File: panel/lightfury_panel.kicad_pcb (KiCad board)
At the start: 6 copper layers, 184.2 x 233.8 mm, 284 parts, among them U1 TLV61070ADBV, U1_2 TLV61070ADBV, U2 SN74LV1T126DBVR, U2_2 SN74LV1T126DBVR

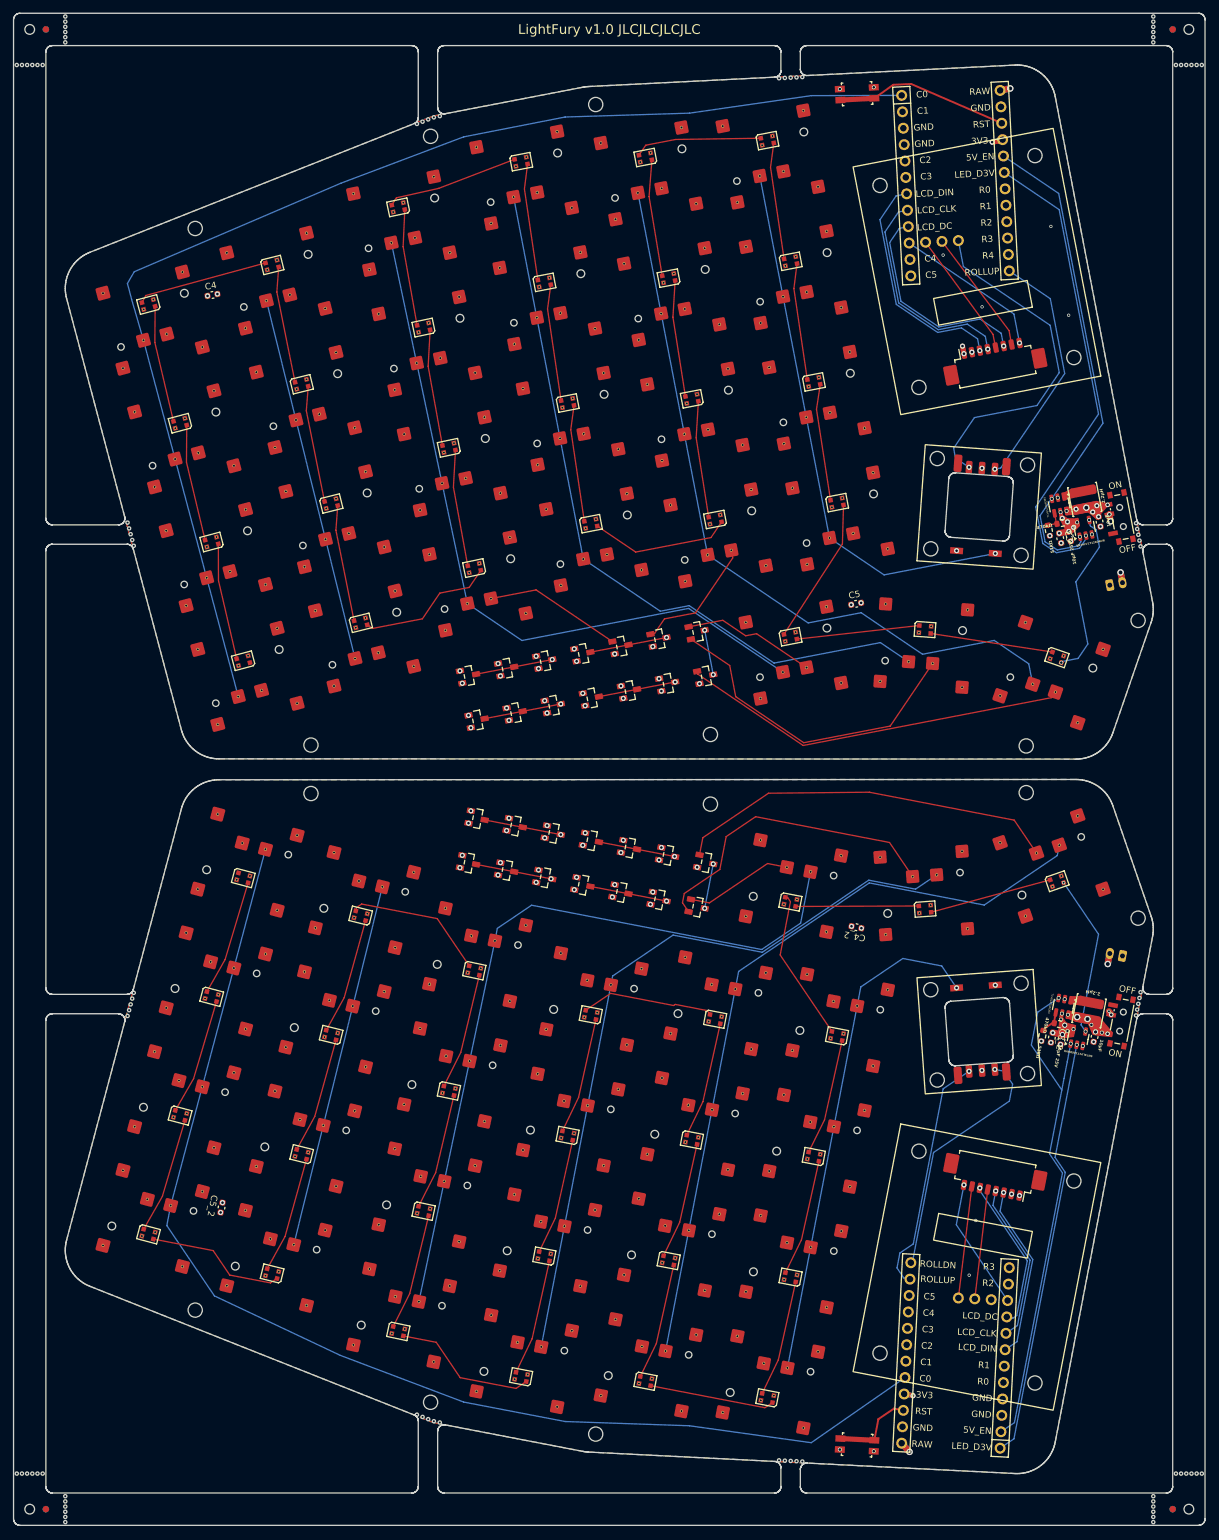
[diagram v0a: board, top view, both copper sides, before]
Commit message: Cleanup
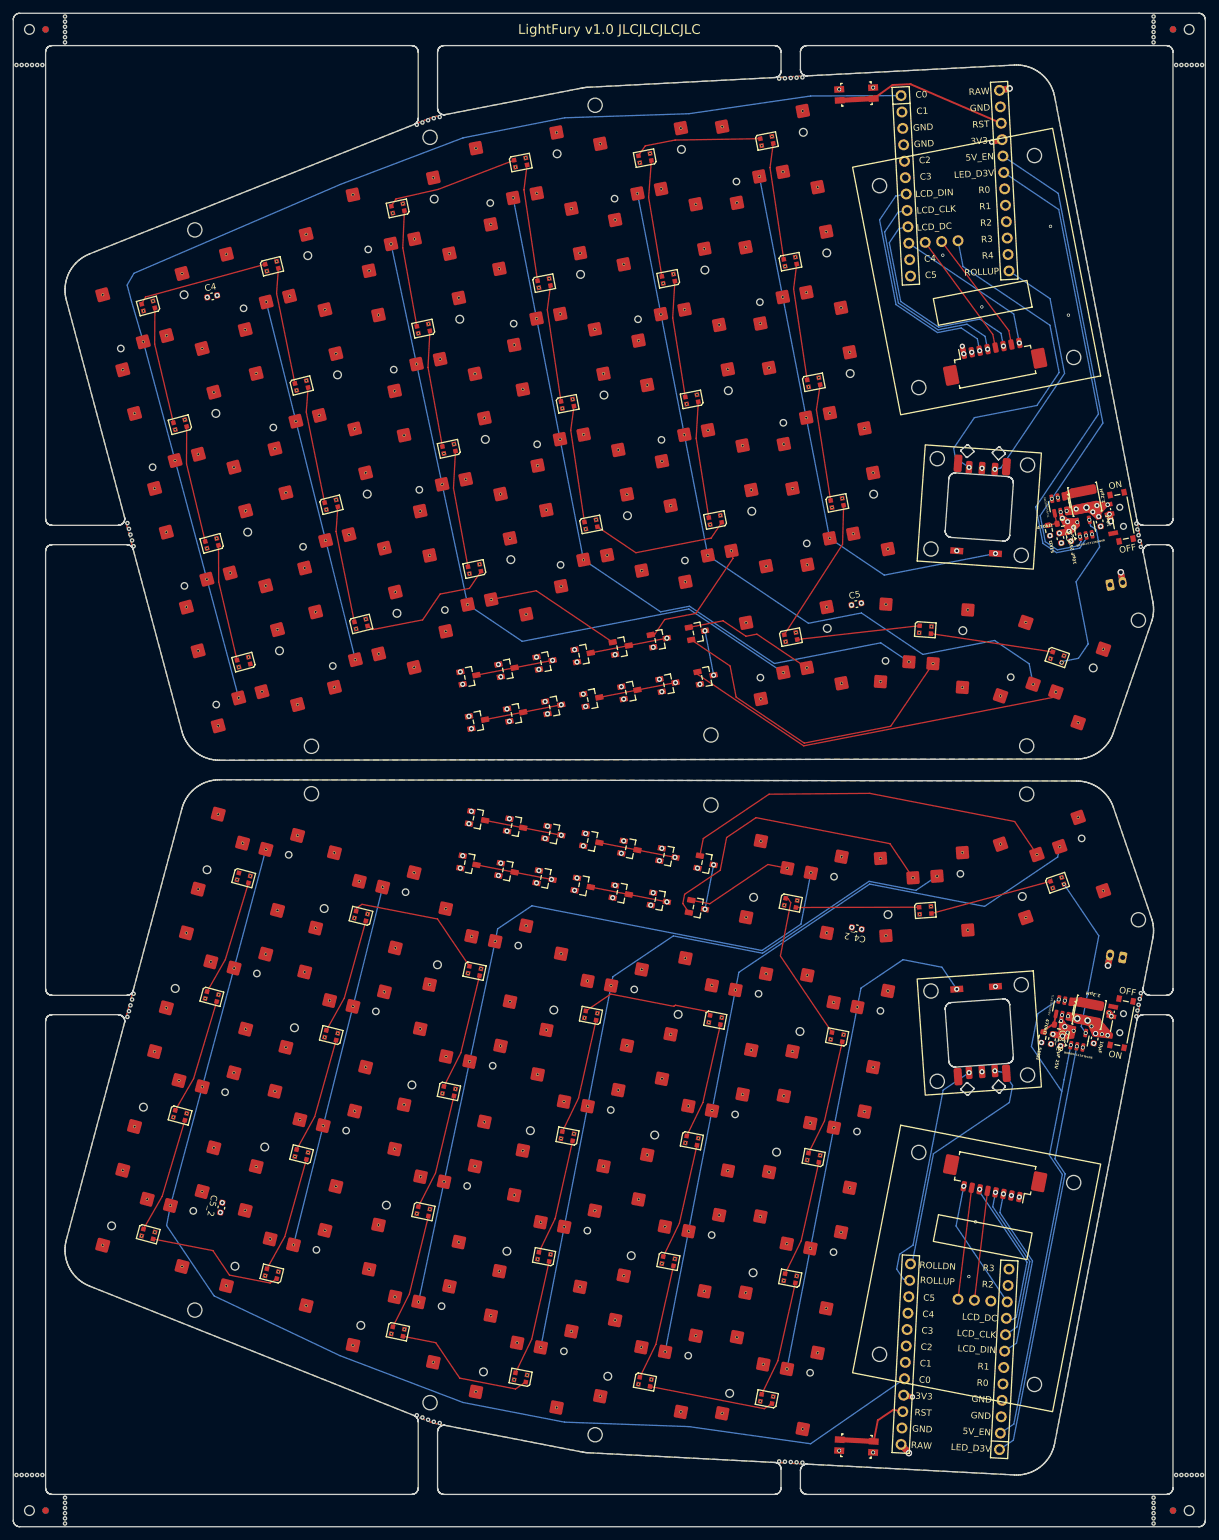
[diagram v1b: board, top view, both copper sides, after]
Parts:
- moved MH7_2 0.26 mm to (230.3, 160.2), turned to -161 degrees
- moved JST1_2 0.25 mm to (226.9, 165.8), turned to -11 degrees
- moved PWR1_2 0.25 mm to (227.7, 176.1), turned to -11 degrees
- moved C1_2 0.24 mm to (223.6, 178.5), turned to -101 degrees
- moved L1_2 0.24 mm to (222.7, 174.5), turned to 79 degrees
- moved LED4 0.24 mm to (77.2, 65.3), turned to -165 degrees
- moved LED15_2 0.24 mm to (217.8, 154.4), turned to 19 degrees
- moved S4 0.24 mm to (77.9, 67.7), turned to 15 degrees
- moved S27_2 0.24 mm to (216.9, 152.1), turned to -161 degrees
- moved U2_2 0.24 mm to (221.0, 178.6), turned to 79 degrees
- moved MH6_2 0.23 mm to (213.0, 140.7), turned to -161 degrees
- moved U1_2 0.23 mm to (218.7, 173.8), turned to -101 degrees
- moved C2_2 0.23 mm to (218.4, 178.9), turned to -101 degrees
- moved R1_2 0.23 mm to (218.1, 176.5), turned to 169 degrees
- moved MH1 0.23 mm to (84.4, 53.5), turned to 15 degrees
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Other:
- board size 184.2 x 233.8 mm -> 184.3 x 234 mm
